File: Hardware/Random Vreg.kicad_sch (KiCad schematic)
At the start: 11 parts, among them J1 Conn_01x07_Male, J2 Conn_01x04_Male, J3 Conn_01x02_Male, J4 Conn_01x02_Male, J5 Conn_01x02_Male, J6 Conn_01x02_Male, J7 Conn_01x08_Male, J9 QWIIC_Stackable, U1 R1501J033B-T1-JE

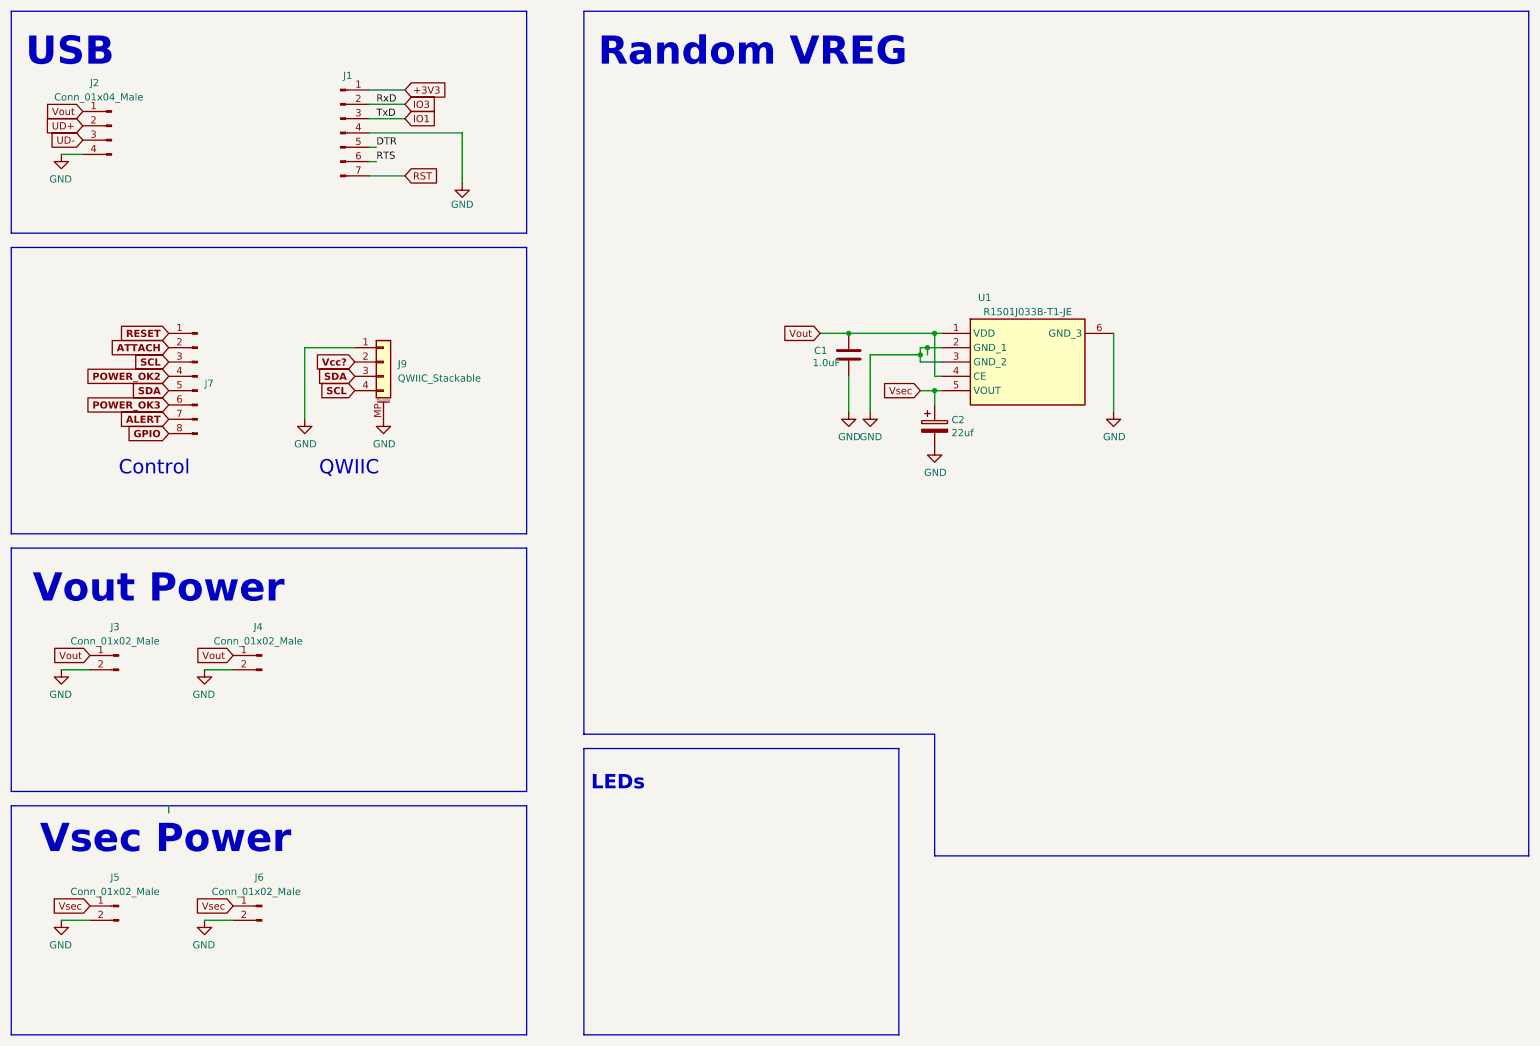
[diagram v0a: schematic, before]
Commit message: ...
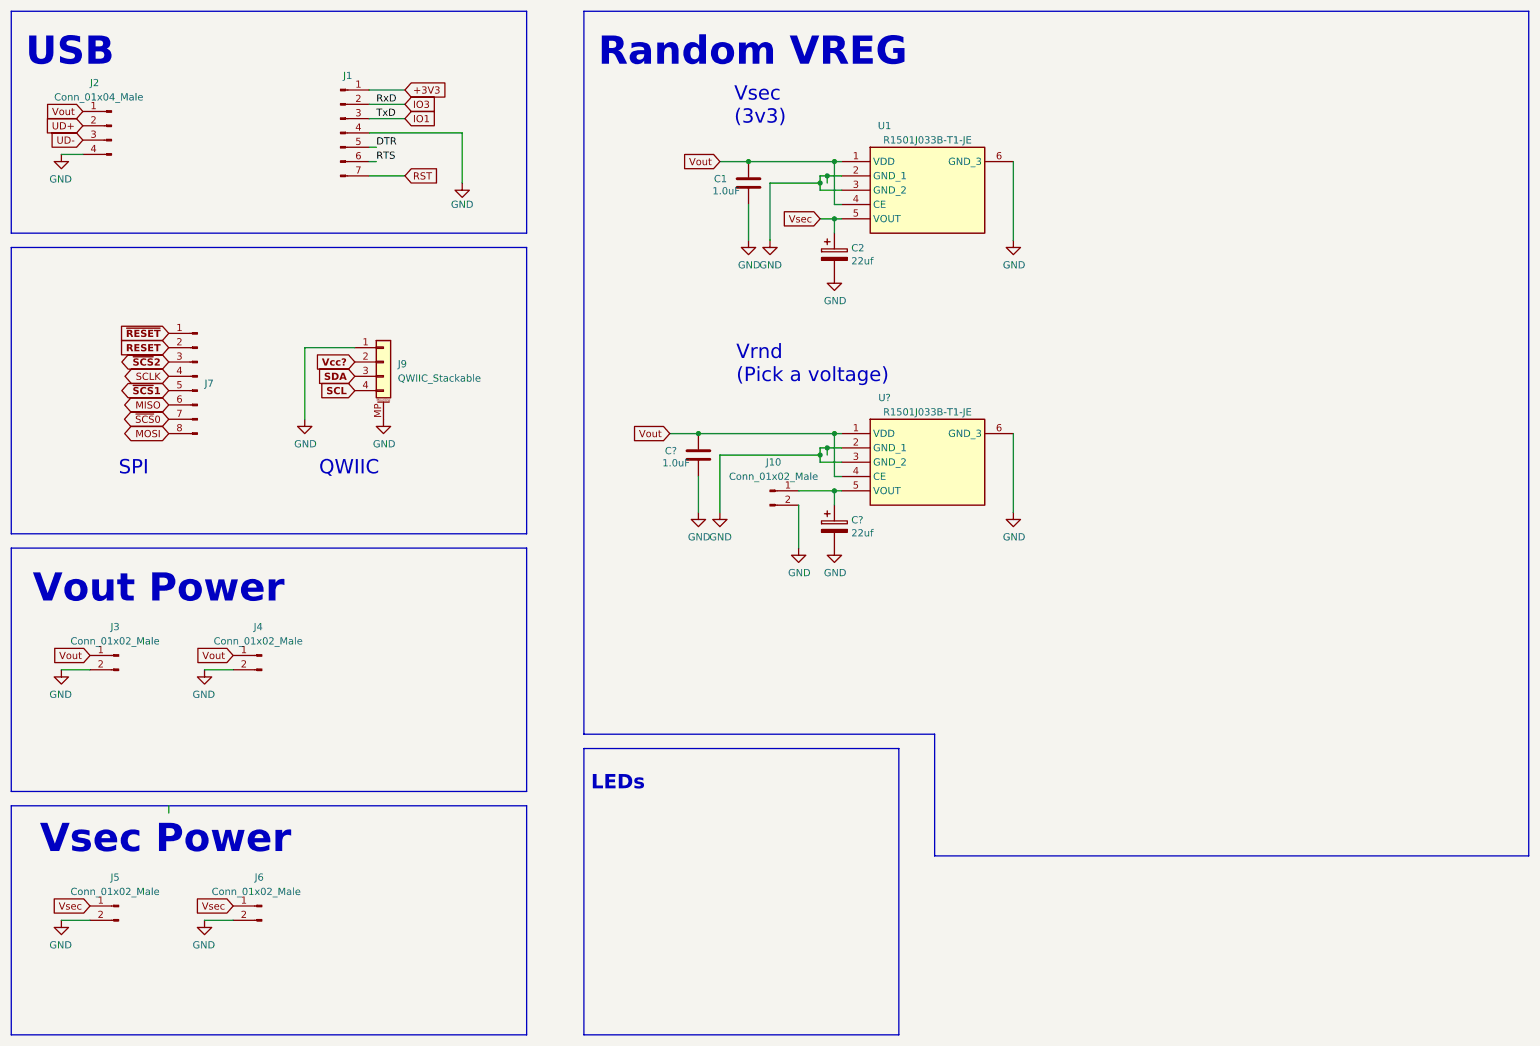
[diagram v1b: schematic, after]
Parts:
- added C?: 1.0uF, Capacitor_SMD:C_0603_1608Metric, symbol Device:C
- added C?: 22uf, Tinker:CP_EIA-6032-28-Tantalumm_HandSolder, symbol Device:CP
- added J10: Conn_01x02_Male, Tinker:Board_Stacker_2, symbol Connector:Conn_01x02_Male
- added U?: R1501J033B-T1-JE, Tinker:R1501J033BT1JE, symbol R1501J033B-T1-JE:R1501J033B-T1-JE
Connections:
- net ATTACH is gone; now on net RESET: J7.2 (Pin_2)
- net GND: now also C?.2, C?.2, J10.2 (Pin_2), U?.2 (GND_1), U?.3 (GND_2), U?.6 (GND_3)
- net RESET: no longer J7.1 (Pin_1)
- net SCL: no longer J7.3 (Pin_3)
- net SDA: no longer J7.5 (Pin_5)
- net Vout: now also C?.1, U?.1 (VDD), U?.4 (CE)
- net ALERT renamed ~{SCS}0
- net GPIO renamed MOSI
- net POWER_OK2 renamed SCLK
- net POWER_OK3 renamed MISO
- new net: C?.1, J10.1 (Pin_1), U?.5 (VOUT)
- new net ~{RESET}: J7.1 (Pin_1)
- new net ~{SCS}1: J7.5 (Pin_5)
- new net ~{SCS}2: J7.3 (Pin_3)
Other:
- note added: "SPI"
- note added: "Vrnd (Pick a voltage)"
- note added: "Vsec (3v3)"
- note removed: "Control"
- moved on the sheet: C1, C2, U1
